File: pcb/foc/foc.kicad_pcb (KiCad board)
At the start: 2 copper layers, 7 parts, among them J1 PH_2.0, J2 TB_MOTOR, J3 Power42V, J4 Conn_01x03_Pin, Q1 BTN8982TA, Q2 BTN8982TA, Q3 BTN8982TA

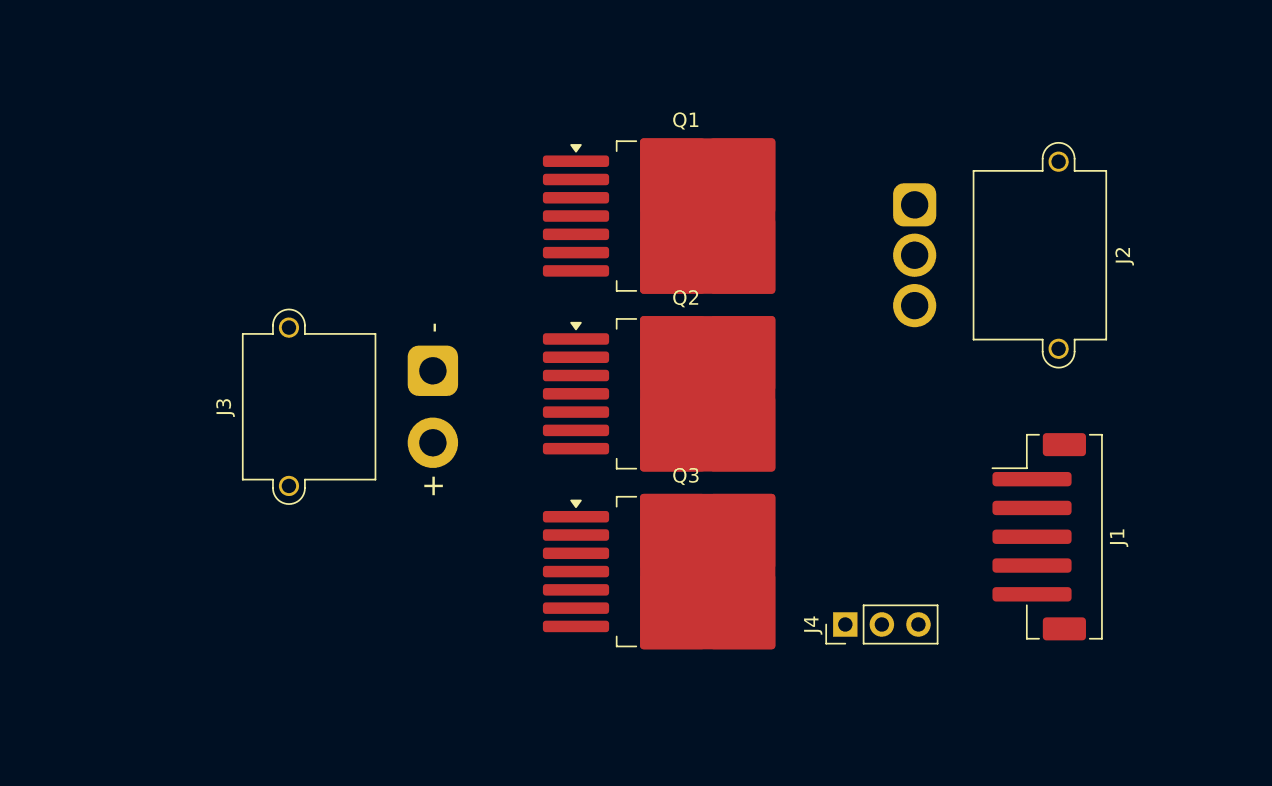
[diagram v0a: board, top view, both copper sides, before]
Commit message: 更新原理图和pcb
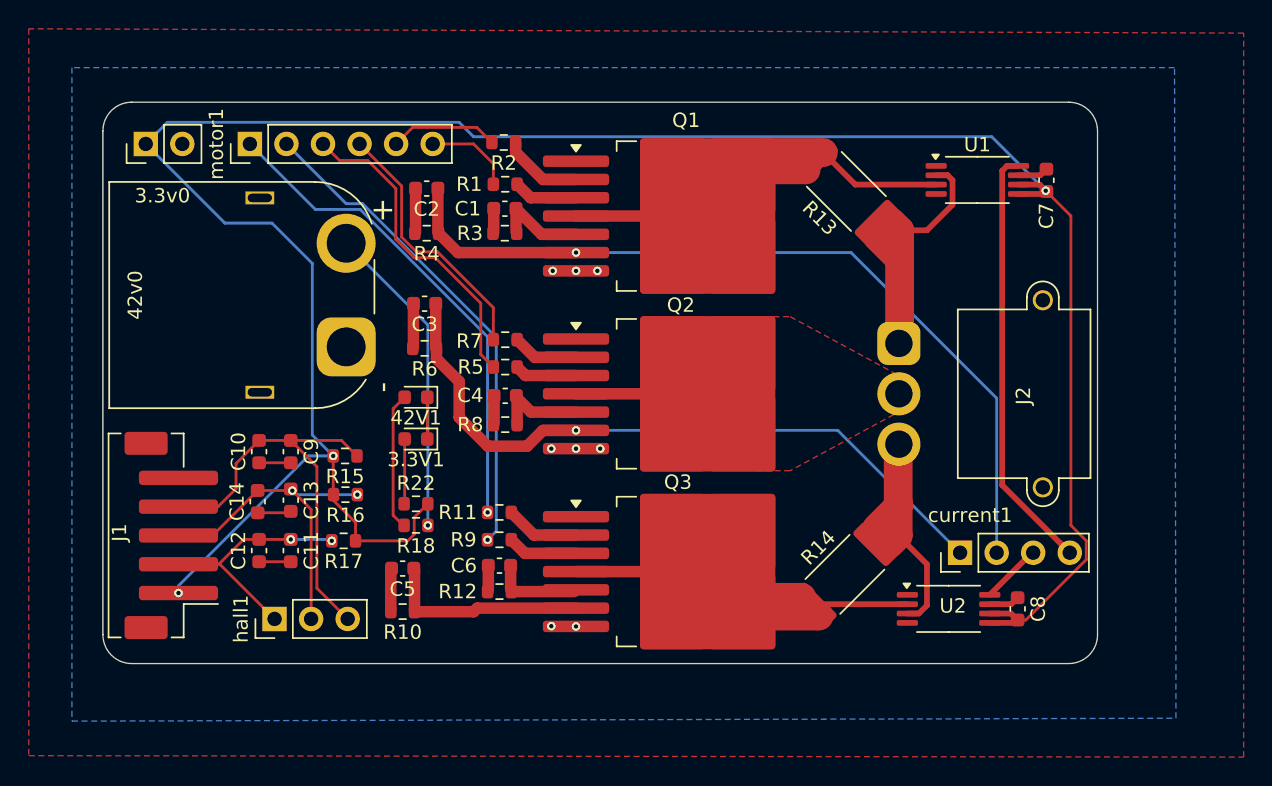
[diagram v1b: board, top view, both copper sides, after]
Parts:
- removed J3: Power42V, Connector_AMASS:AMASS_XT30PW-M_1x02_P2.50mm_Horizontal
- removed J4: Conn_01x03_Pin, Connector_PinHeader_2.54mm:PinHeader_1x03_P2.54mm_Vertical
- added 3.3V1: LED, LED_SMD:LED_0603_1608Metric, F.Cu at (118.0, 91.0)
- added 3.3v0: Power3.3, Connector_PinHeader_2.54mm:PinHeader_1x02_P2.54mm_Vertical, F.Cu at (99.2, 70.5)
- added 42V1: LED, LED_SMD:LED_0603_1608Metric, F.Cu at (118.0, 88.1)
- added 42v0: Power42V, Connector_AMASS:AMASS_XT60PW-M_1x02_P7.20mm_Horizontal, F.Cu at (113.2, 84.6)
- added C1: 100nF, Capacitor_SMD:C_0603_1608Metric, F.Cu at (124.2, 75.0)
- added C10: 20pF, Capacitor_SMD:C_0603_1608Metric, F.Cu at (107.1, 91.9)
- added C11: 100nF, Capacitor_SMD:C_0603_1608Metric, F.Cu at (109.3, 98.8)
- added C12: 20pF, Capacitor_SMD:C_0603_1608Metric, F.Cu at (107.1, 98.8)
- added C13: 100nF, Capacitor_SMD:C_0603_1608Metric, F.Cu at (109.3, 95.2)
- added C14: 20pF, Capacitor_SMD:C_0603_1608Metric, F.Cu at (107.0, 95.3)
- added C2: 1nF, Capacitor_SMD:C_0603_1608Metric, F.Cu at (118.7, 73.6)
- added C3: 1nF, Capacitor_SMD:C_0603_1608Metric, F.Cu at (118.6, 81.6)
- added C4: 100nF, Capacitor_SMD:C_0603_1608Metric, F.Cu at (124.2, 88.0)
- added C5: 1nF, Capacitor_SMD:C_0603_1608Metric, F.Cu at (117.1, 100.0)
- added C6: 100nF, Capacitor_SMD:C_0603_1608Metric, F.Cu at (123.8, 99.8)
- added C7: 0.1nF, Capacitor_SMD:C_0603_1608Metric, F.Cu at (161.8, 73.0)
- added C8: 0.1nF, Capacitor_SMD:C_0603_1608Metric, F.Cu at (159.8, 102.8)
- added C9: 100nF, Capacitor_SMD:C_0603_1608Metric, F.Cu at (109.3, 91.9)
- added NT1: NetTie_2, NetTie:NetTie-2_SMD_Pad2.0mm, F.Cu at (144.0, 103.3)
- added NT1: NetTie_2, NetTie:NetTie-2_SMD_Pad2.0mm, F.Cu at (142.8, 102.0)
- added NT2: NetTie_2, NetTie:NetTie-2_SMD_Pad2.0mm, F.Cu at (151.5, 93.4)
- added NT3: NetTie_2, NetTie:NetTie-2_SMD_Pad2.0mm, F.Cu at (151.6, 82.4)
- added NT4: NetTie_2, NetTie:NetTie-2_SMD_Pad2.0mm, F.Cu at (144.3, 71.1)
- added NT4: NetTie_2, NetTie:NetTie-2_SMD_Pad2.0mm, F.Cu at (143.1, 72.3)
- added R1: 10k, Resistor_SMD:R_0603_1608Metric, F.Cu at (124.2, 73.3)
- added R10: 1k, Resistor_SMD:R_0603_1608Metric, F.Cu at (117.1, 103.0)
- added R11: 10k, Resistor_SMD:R_0603_1608Metric, F.Cu at (123.8, 96.1)
- added R12: 0.51k, Resistor_SMD:R_0603_1608Metric, F.Cu at (123.8, 101.6)
- added R13: 0.001, Resistor_SMD:R_2512_6332Metric, F.Cu at (147.9, 73.8)
- added R14: 0.001, Resistor_SMD:R_2512_6332Metric, F.Cu at (147.8, 100.4)
- added R15: 3.3k, Resistor_SMD:R_0603_1608Metric, F.Cu at (113.1, 92.2)
- added R16: 3.3k, Resistor_SMD:R_0603_1608Metric, F.Cu at (113.1, 94.9)
- added R17: 3.3k, Resistor_SMD:R_0603_1608Metric, F.Cu at (113.0, 98.1)
- added R18: 10k, Resistor_SMD:R_0603_1608Metric, F.Cu at (118.0, 97.0)
- added R2: 10k, Resistor_SMD:R_0603_1608Metric, F.Cu at (124.1, 70.4)
- added R22: 1k, Resistor_SMD:R_0603_1608Metric, F.Cu at (118.0, 95.5)
- added R3: 0.51k, Resistor_SMD:R_0603_1608Metric, F.Cu at (124.2, 76.7)
- added R4: 1k, Resistor_SMD:R_0603_1608Metric, F.Cu at (118.7, 76.7)
- added R5: 10k, Resistor_SMD:R_0603_1608Metric, F.Cu at (124.2, 86.0)
- added R6: 1k, Resistor_SMD:R_0603_1608Metric, F.Cu at (118.6, 84.7)
- added R7: 10k, Resistor_SMD:R_0603_1608Metric, F.Cu at (124.2, 84.1)
- added R8: 0.51k, Resistor_SMD:R_0603_1608Metric, F.Cu at (124.2, 90.0)
- added R9: 10k, Resistor_SMD:R_0603_1608Metric, F.Cu at (123.8, 98.0)
- added U1: INA240A2PW, Package_SO:TSSOP-8_4.4x3mm_P0.65mm, F.Cu at (157.0, 73.0)
- added U2: INA240A2PW, Package_SO:TSSOP-8_4.4x3mm_P0.65mm, F.Cu at (155.0, 102.8)
- added current1: current info, Connector_PinHeader_2.54mm:PinHeader_1x04_P2.54mm_Vertical, F.Cu at (155.8, 98.9)
- added hall1: hall sig, Connector_PinHeader_2.54mm:PinHeader_1x03_P2.54mm_Vertical, F.Cu at (108.2, 103.5)
- added motor1: sig in, Connector_PinHeader_2.54mm:PinHeader_1x06_P2.54mm_Vertical, F.Cu at (106.5, 70.5)
- moved J1 60.3 mm to (101.0, 97.7), turned to 90 degrees
- moved J2 9.69 mm to (151.6, 84.4)
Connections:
- J1 pad 1: VCC -> +3.3V
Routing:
- net +3.3V: track 0.00 -> 163.8 mm, vias 0 -> 3
- net A2: track 0.00 -> 57.4 mm, vias 0 -> 1
- net A3: track 0.00 -> 48.2 mm, vias 0 -> 1
- net D5: track 0.00 -> 34.5 mm, vias 0 -> 1
- net D4: track 0.00 -> 34.3 mm, vias 0 -> 1
- net VCC: track 0.00 -> 30.5 mm, vias 0 -> 9
- net MOT_C: track 0.00 -> 29.8 mm
- net A0: track 0.00 -> 29.8 mm
- net GND: track 0.00 -> 24.4 mm
- net MOT_B: track 0.00 -> 23.4 mm, vias 0 -> 2
- net D6: track 0.00 -> 22.4 mm
- net MOT_A: track 0.00 -> 19.7 mm, vias 0 -> 2
- net D7: track 0.00 -> 18.3 mm
- net Net-(U1-+): track 0.00 -> 14.4 mm
- net Net-(Q3-IS): track 0.00 -> 14.3 mm
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- added copper zone on F.Cu, net GND
- added copper zone on B.Cu, net VCC
- added copper zone on F.Cu, net out2
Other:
- board outline added: 69.1 x 39 mm
